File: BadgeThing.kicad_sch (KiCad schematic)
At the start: 61 parts, among them J2 Ext 5V, J3 External 3V3, J4 SWD Header, J5 USB_C_Receptacle_USB2.0, J6 Connector_Generic_Conn_01x02, J7 Conn_01x06, SW1 ESP RESET, SW2 Left, SW3 Down, SW4 Select, SW5 Up, SW6 Right, SW7 BOOTSEL, U1 ESP-12F, U3 RP2040, U4 NCP1117-3.3_SOT223, U5 W25Q32JVSS, U6 USBLC6-2SC6, Y1 12.000MHz

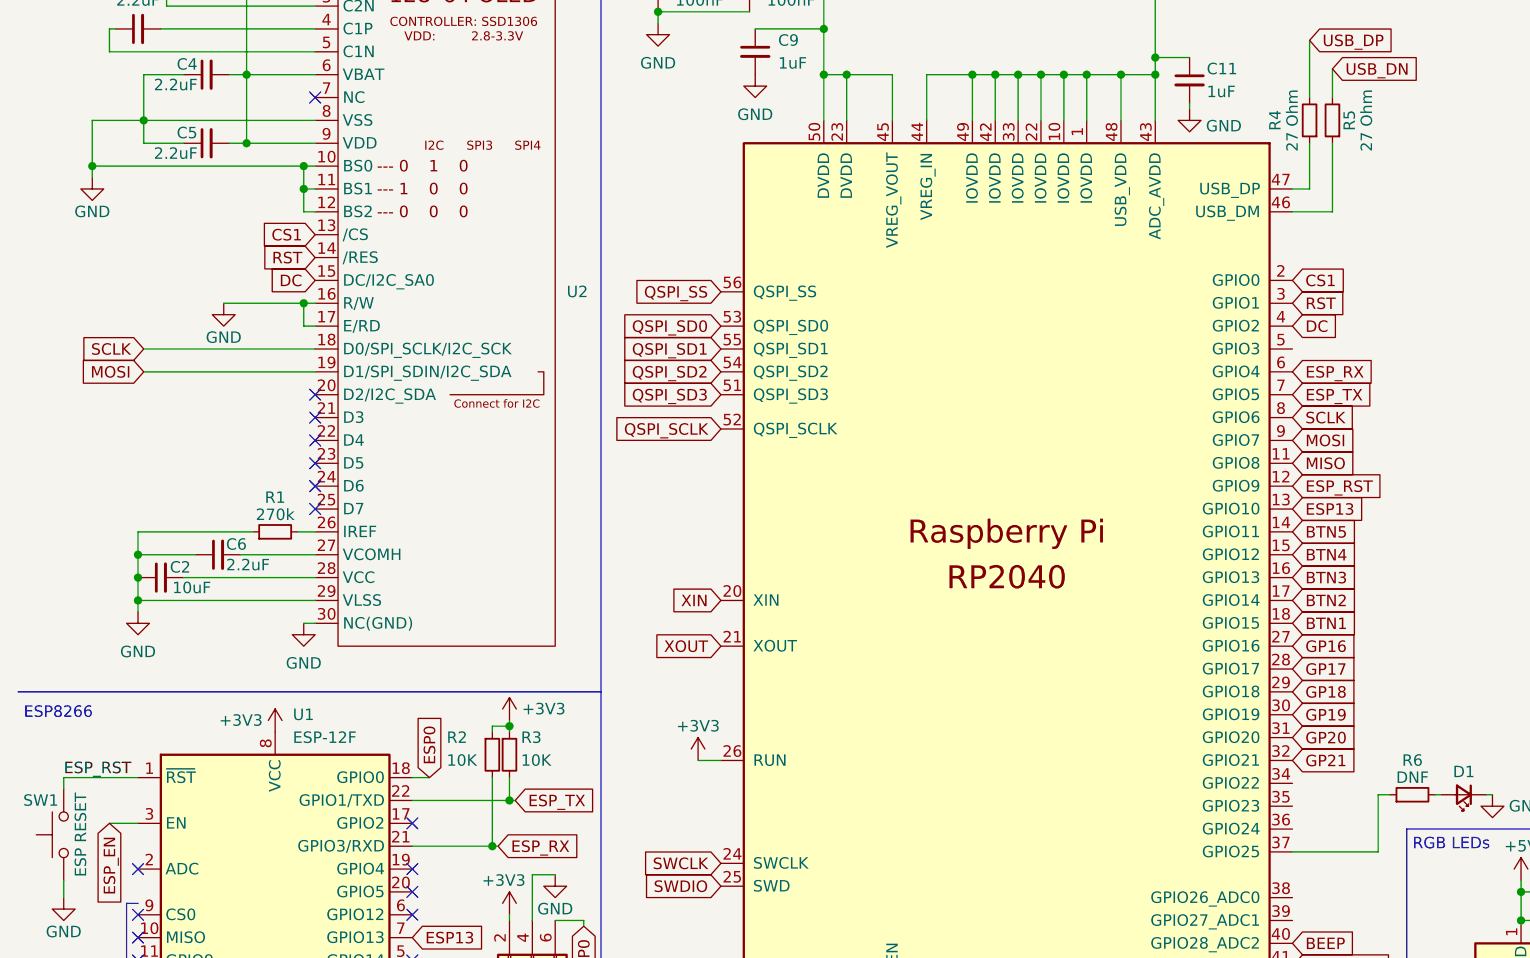
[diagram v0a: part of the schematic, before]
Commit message: Final routing
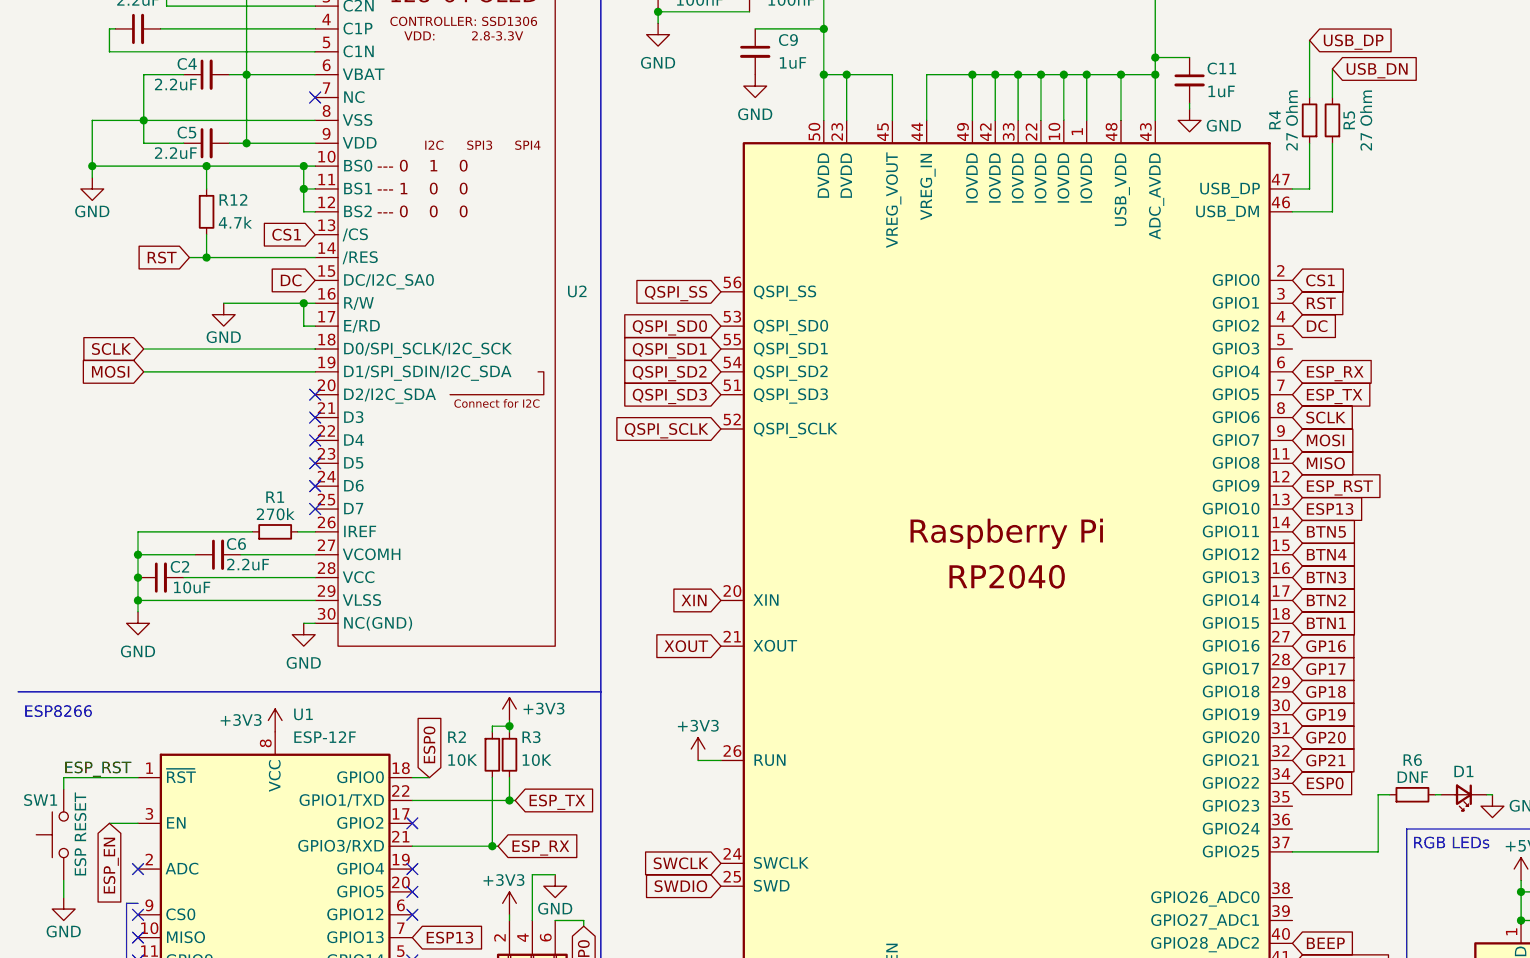
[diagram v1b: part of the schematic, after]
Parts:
- added R12: 4.7k, Resistor_SMD:R_0402_1005Metric_Pad0.72x0.64mm_HandSolder, symbol Device:R_Small
- U6: LCSC C111212 -> C2687116
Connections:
- net ESP0: now also U3.34 (GPIO22)
- net GND: now also R12.1
- net RST: now also R12.2
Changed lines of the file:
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@@
   (junction (at 25.4 88.9) (diameter 0) (color 0 0 0 0)
   )
+  (junction (at 33.02 45.72) (diameter 0) (color 0 0 0 0)
+  )
   (junction (at 201.93 74.93) (diameter 0) (color 0 0 0 0)
   )
@@
   (junction (at 179.07 126.365) (diameter 0) (color 0 0 0 0)
   )
+  (junction (at 33.02 55.88) (diameter 0) (color 0 0 0 0)
+  )
   (junction (at 243.205 38.735) (diameter 0) (color 0 0 0 0)
   )
@@
     (stroke (width 0) (type default))
   )
+  (wire (pts (xy 31.115 55.88) (xy 33.02 55.88))
+    (stroke (width 0) (type default))
+  )
   (wire (pts (xy 162.56 19.05) (xy 172.72 19.05))
     (stroke (width 0) (type default))
@@
     (stroke (width 0) (type default))
   )
+  (wire (pts (xy 33.02 45.72) (xy 33.02 48.26))
+    (stroke (width 0) (type default))
+  )
   (wire (pts (xy 238.125 55.88) (xy 238.125 55.245))
     (stroke (width 0) (type default))
@@
     (stroke (width 0) (type default))
   )
+  (wire (pts (xy 33.02 45.72) (xy 43.815 45.72))
+    (stroke (width 0) (type default))
+  )
   (polyline (pts (xy 191.516 34.925) (xy 193.167 34.925))
     (stroke (width 0) (type default))
@@
     (stroke (width 0) (type default))
   )
+  (wire (pts (xy 33.02 55.88) (xy 45.085 55.88))
+    (stroke (width 0) (type default))
+  )
   (wire (pts (xy 227.965 74.93) (xy 227.965 84.455))
     (stroke (width 0) (type default))
@@
     (stroke (width 0) (type default))
   )
-  (wire (pts (xy 20.32 45.72) (xy 43.815 45.72))
-    (stroke (width 0) (type default))
-  )
   (wire (pts (xy 43.815 60.96) (xy 43.815 63.5))
     (stroke (width 0) (type default))
@@
     (stroke (width 0) (type default))
   )
+  (wire (pts (xy 33.02 53.34) (xy 33.02 55.88))
+    (stroke (width 0) (type default))
+  )
   (polyline (pts (xy 263.525 153.67) (xy 284.988 153.67))
     (stroke (width 0) (type default))
@@
     (stroke (width 0) (type default))
   )
+  (wire (pts (xy 20.32 45.72) (xy 33.02 45.72))
+    (stroke (width 0) (type default))
+  )
   (wire (pts (xy 74.295 163.83) (xy 73.025 163.83))
     (stroke (width 0) (type default))
@@
     )
   )
+  (global_label "ESP0" (shape input) (at 153.67 114.3 0) (fields_autoplaced)
+    (effects (font (size 1.27 1.27)) (justify left))
+    (property "Intersheetrefs" "${INTERSHEET_REFS}" (at 161.4138 114.3 0)
+      (effects (font (size 1.27 1.27)) (justify left) hide)
+    )
+  )
   (global_label "ESP13" (shape input) (at 153.67 83.82 0) (fields_autoplaced)
     (effects (font (size 1.27 1.27)) (justify left))
@@
     )
   )
-  (global_label "RST" (shape input) (at 45.085 55.88 180) (fields_autoplaced)
+  (global_label "RST" (shape input) (at 31.115 55.88 180) (fields_autoplaced)
     (effects (font (size 1.27 1.27)) (justify right))
-    (property "Intersheetrefs" "${INTERSHEET_REFS}" (at 38.7321 55.88 0)
+    (property "Intersheetrefs" "${INTERSHEET_REFS}" (at 24.7621 55.88 0)
       (effects (font (size 1.27 1.27)) (justify right) hide)
     )
@@
       (effects (font (size 1.27 1.27)) hide)
     )
-    (property "LCSC" "C111212" (at 99.695 170.18 0)
+    (property "LCSC" "C2687116" (at 99.695 170.18 0)
       (effects (font (size 1.27 1.27)) hide)
     )
@@
         )
       )
+    )
+  )
+  (symbol (lib_id "Device:R_Small") (at 33.02 50.8 0) (unit 1)
+    (in_bom yes) (on_board yes) (dnp no)
+    (property "Reference" "R12" (at 34.29 49.53 0)
+      (effects (font (size 1.27 1.27)) (justify left))
+    )
+    (property "Value" "4.7k" (at 34.29 52.07 0)
+      (effects (font (size 1.27 1.27)) (justify left))
+    )
+    (property "Footprint" "Resistor_SMD:R_0402_1005Metric_Pad0.72x0.64mm_HandSolder" (at 33.02 50.8 0)
+      (effects (font (size 1.27 1.27)) hide)
+    )
+    (property "Datasheet" "~" (at 33.02 50.8 0)
+      (effects (font (size 1.27 1.27)) hide)
+    )
+    (property "LCSC" "C25900" (at 33.02 50.8 0)
+      (effects (font (size 1.27 1.27)) hide)
+    )
+    (pin "1")
+    (pin "2")
+    (instances
+      (project "BadgeThing"
+        (path "/35d5f6bf-e39e-48ab-813a-17587fce37db"
+          (reference "R12") (unit 1)
+        )
+      )
